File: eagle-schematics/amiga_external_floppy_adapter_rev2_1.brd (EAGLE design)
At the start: 47 x 51.1 mm, 15 parts, among them IC1 74LS00N, IC2 74LS74N, J1 Computer, J2 Floppy, J3 PINHD-1X4, J4 Passthrough

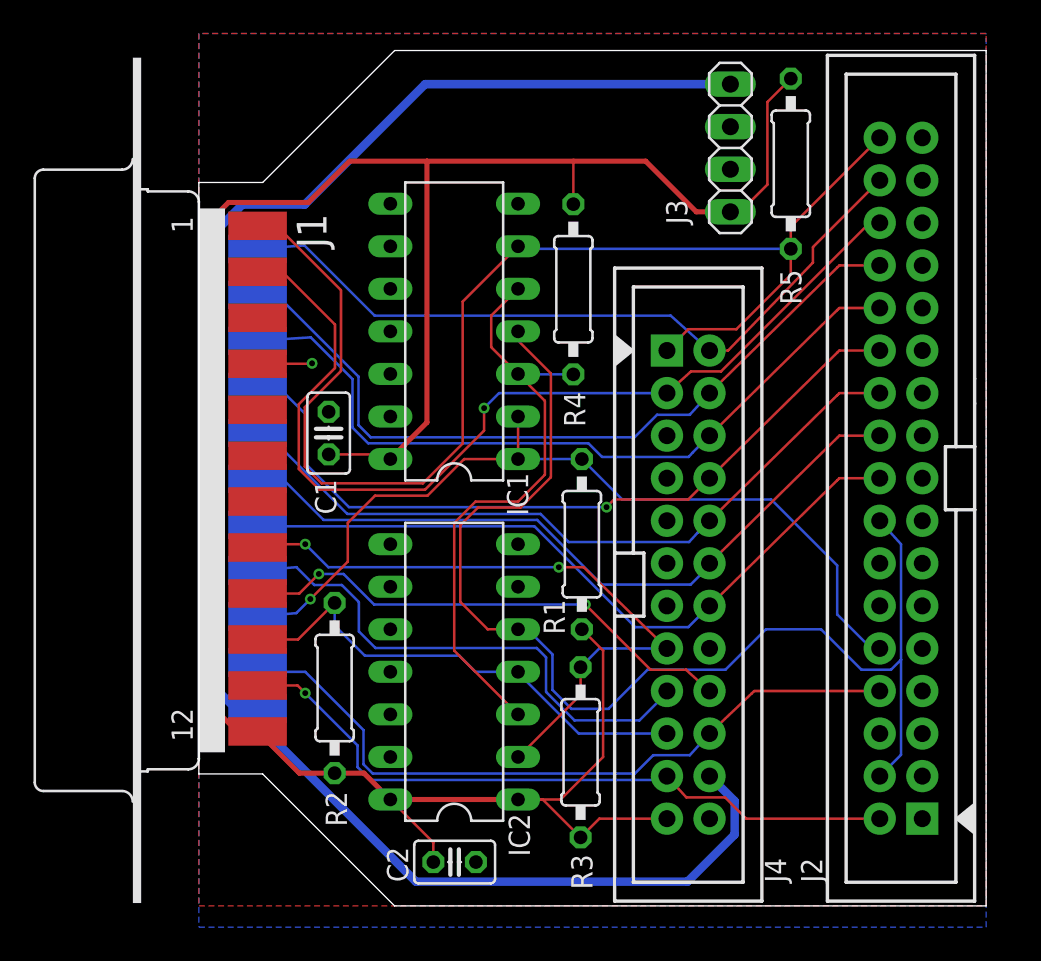
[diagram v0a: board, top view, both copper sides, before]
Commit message: Files for rev2.1 are updated/added, readme file modified slightly
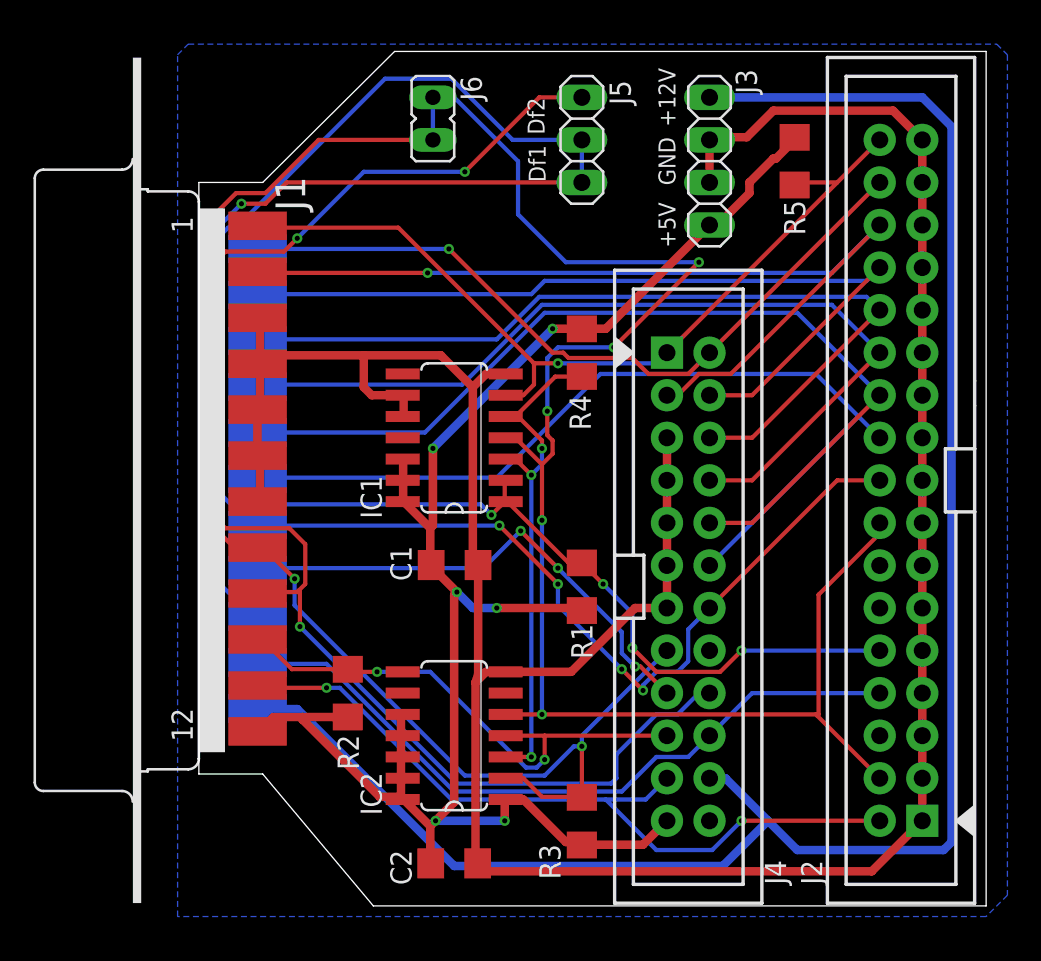
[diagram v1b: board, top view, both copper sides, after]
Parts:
- added J5: (no value), pinhead:1X03
- added J6: (no value), jumper:JP1
- C1, C2: device rcl:C025-025X050 -> rcl:C1206
- IC1: value 74LS00N -> 74LS00D; device 74xx-eu:DIL14 -> 74xx-eu:SO14
- IC2: value 74LS74N -> 74LS74D; device 74xx-eu:DIL14 -> 74xx-eu:SO14
- J3: value PINHD-1X4 -> Power
- R1, R2, R3, R4, R5: device rcl:0207/10 -> rcl:R1206
- moved U$1 15.9 mm to (10.4, 28.7)
- moved C1 10.9 mm to (15.3, 20.3), turned to 0 degrees
- moved IC1 6.35 mm to (15.2, 27.9)
- moved R3 4.12 mm to (22.9, 5.05)
- moved R4 3.82 mm to (22.9, 33.0)
- moved IC2 3.81 mm to (15.2, 10.2)
- moved R1 2.54 mm to (22.9, 19.1)
- moved J3 1.47 mm to (30.5, 44.5)
- moved U$2 0.95 mm to (26.0, 38.4)
- moved R2 0.84 mm to (8.89, 12.7)
- moved R5 0.27 mm to (35.6, 44.5)
- moved J2 0.13 mm to (41.9, 10.2)
- moved J4 0.13 mm to (29.2, 19.1)
- moved C2 0.08 mm to (15.2, 2.54)
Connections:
- new net !SEL: IC1.1, IC1.2, J2.10, J5.2, R1.1
- net !MTR: now also J6.1
- net !MTRX: now also J6.2
- net !SEL1: now also J5.3; no longer IC1.1, IC1.2, J2.10, R1.1
- net !SEL2: now also J5.1
- net +5V: now also IC1.12, IC1.13, IC2.10, IC2.11, IC2.12, IC2.13
- net GND: now also IC1.10, IC1.9
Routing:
- net GND: track 3.26 -> 170.9 mm, vias 1 -> 0
- net !SEL: track 0.00 -> 92.0 mm, vias 0 -> 4
- net !SEL2: track 30.3 -> 86.2 mm, vias 2 -> 3
- net +5V: track 147.2 -> 106.3 mm, vias 0 -> 6
- net !MTRX: track 39.6 -> 79.4 mm
- net !MTR: track 70.3 -> 96.9 mm, vias 0 -> 5
- net !RDY: track 77.9 -> 52.0 mm, vias 0 -> 1
- net !DKWD: track 43.5 -> 55.4 mm
- net !STEP: track 43.6 -> 53.9 mm
- net !DKWE: track 45.8 -> 53.7 mm, vias 1 -> 0
- net +12V: track 103.1 -> 109.8 mm
- net !TK0: track 45.4 -> 51.9 mm
- net !DIR: track 43.3 -> 48.5 mm, vias 0 -> 4
- net N$1: track 36.0 -> 30.9 mm, vias 0 -> 3
- net !CHNG: track 41.5 -> 46.1 mm, vias 1 -> 2
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- removed copper zone on layer 1, net GND
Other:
- board size 47 x 51.1 mm -> 47 x 51 mm
- board text added: "+12V"
- board text added: "+5V"
- board text added: "Cut to Df select"
- board text added: "Df1"
- board text added: "Df2"
- board text added: "Floppy: Open"
- board text added: "GND"
- board text added: "Gotek: Close"
- board text added: "Rev 2.1 - No SMD for Gotek"
- board text added: "mod by Sanyi 2020"
- board text removed: "Rev 2"
